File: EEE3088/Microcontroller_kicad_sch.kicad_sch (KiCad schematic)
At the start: 9 parts, among them J1 MICROXNJ, U1 STM32F051C6Tx, U2 CH340G, U3 AT24C256C-SSHL-T

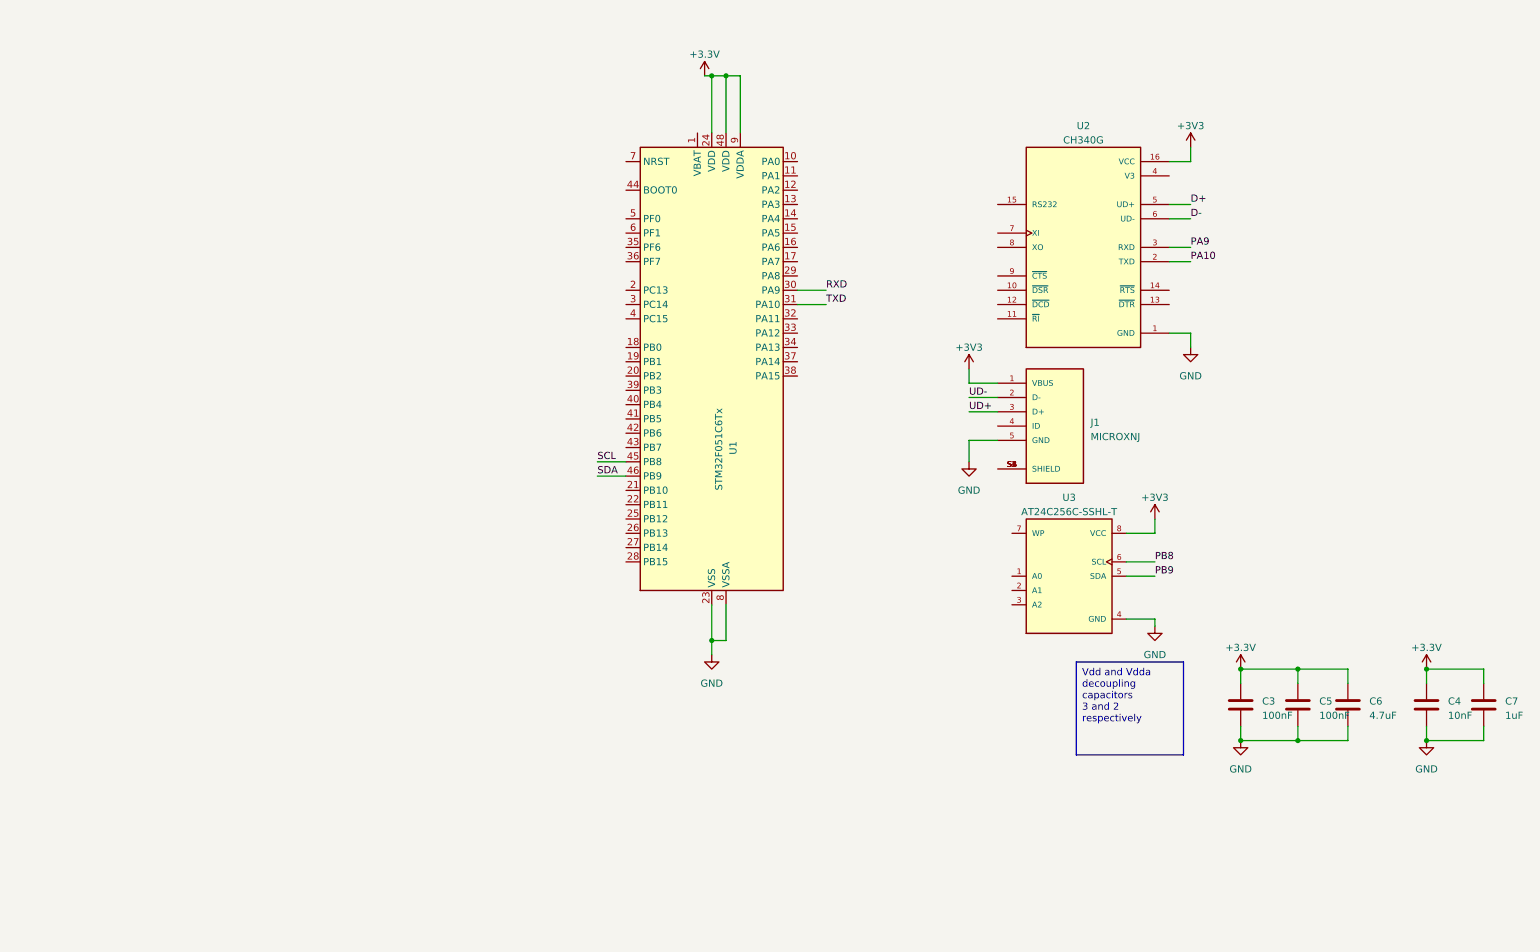
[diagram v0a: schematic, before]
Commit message: 05/03
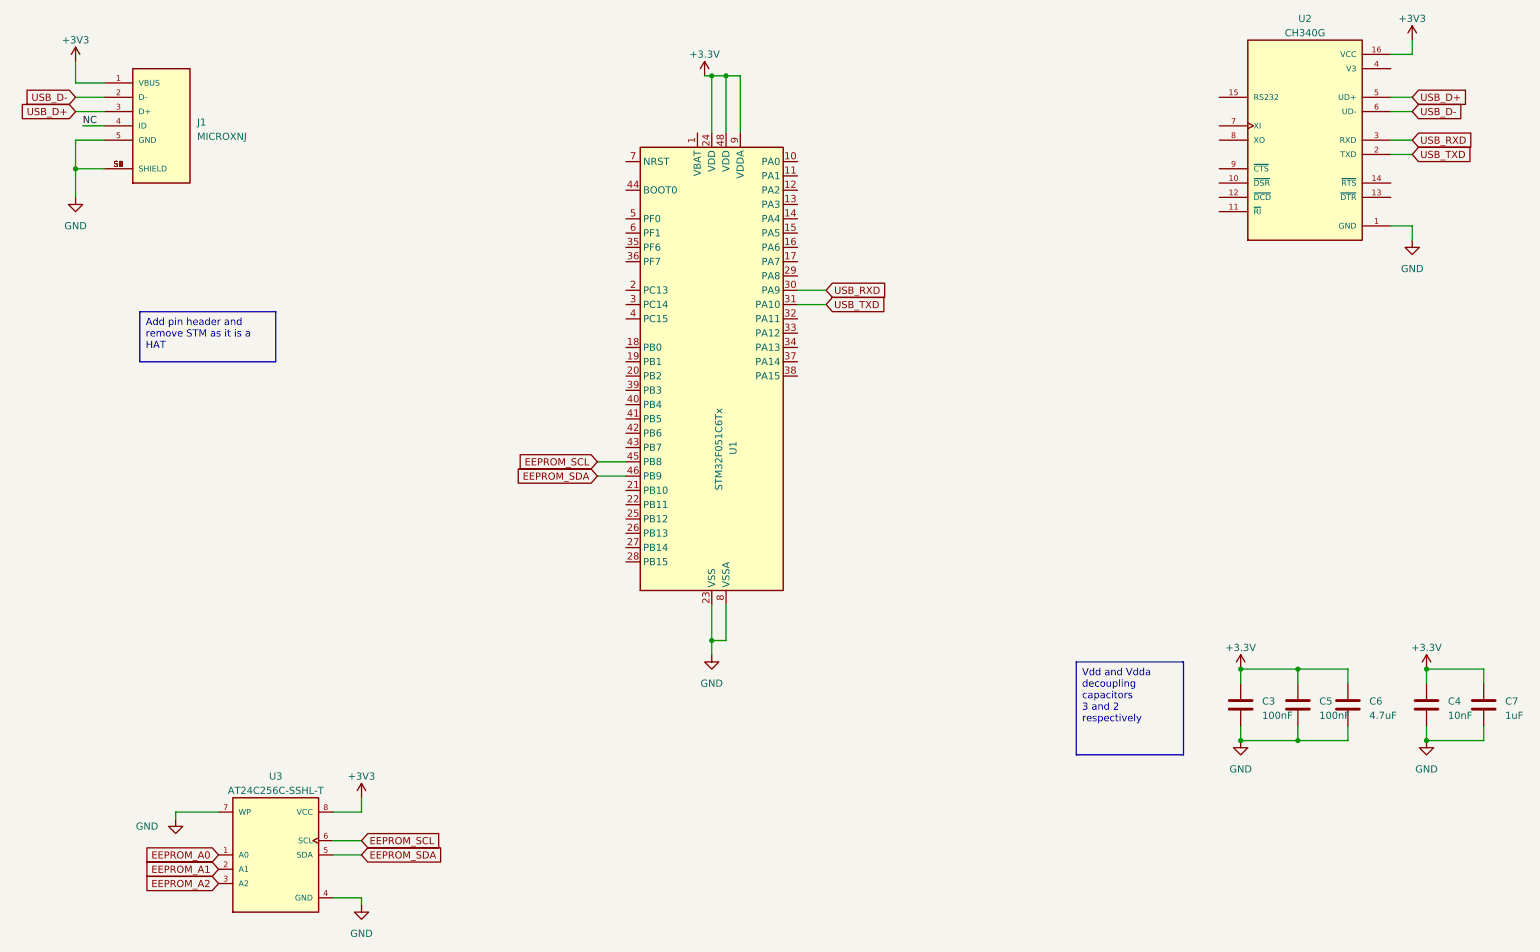
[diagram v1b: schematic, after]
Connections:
- net RXD is gone; now on net USB_RXD: U1.30 (PA9)
- net SCL is gone; now on net EEPROM_SCL: U1.45 (PB8)
- net SDA is gone; now on net EEPROM_SDA: U1.46 (PB9)
- net TXD is gone; now on net USB_TXD: U1.31 (PA10)
- net UD+ is gone; now on net USB_D+: J1.3 (D+)
- net UD- is gone; now on net USB_D-: J1.2 (D-)
- net GND: now also J1.S1 (SHIELD), J1.S2 (SHIELD), J1.S3 (SHIELD), J1.S4 (SHIELD), J1.S5 (SHIELD), J1.S6 (SHIELD), U3.7 (WP)
- net EEPROM_A0: now reaches U3.1 (A0)
- net EEPROM_A1: now reaches U3.2 (A1)
- net EEPROM_A2: now reaches U3.3 (A2)
- net NC: now reaches J1.4 (ID)
- net D+ renamed USB_D+
- net D- renamed USB_D-
- net PA10 renamed USB_TXD
- net PA9 renamed USB_RXD
- net PB8 renamed EEPROM_SCL
- net PB9 renamed EEPROM_SDA
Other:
- moved on the sheet: J1, U2, U3
